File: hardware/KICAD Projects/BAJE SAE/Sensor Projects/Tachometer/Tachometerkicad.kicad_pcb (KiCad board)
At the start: 2 copper layers, 81 x 89 mm, 26 parts, among them J1 Conn_01x02, J3 Conn_01x02, J4 CAN to outer connector, Q1 NPN, U1 NE555P, U2 LM311

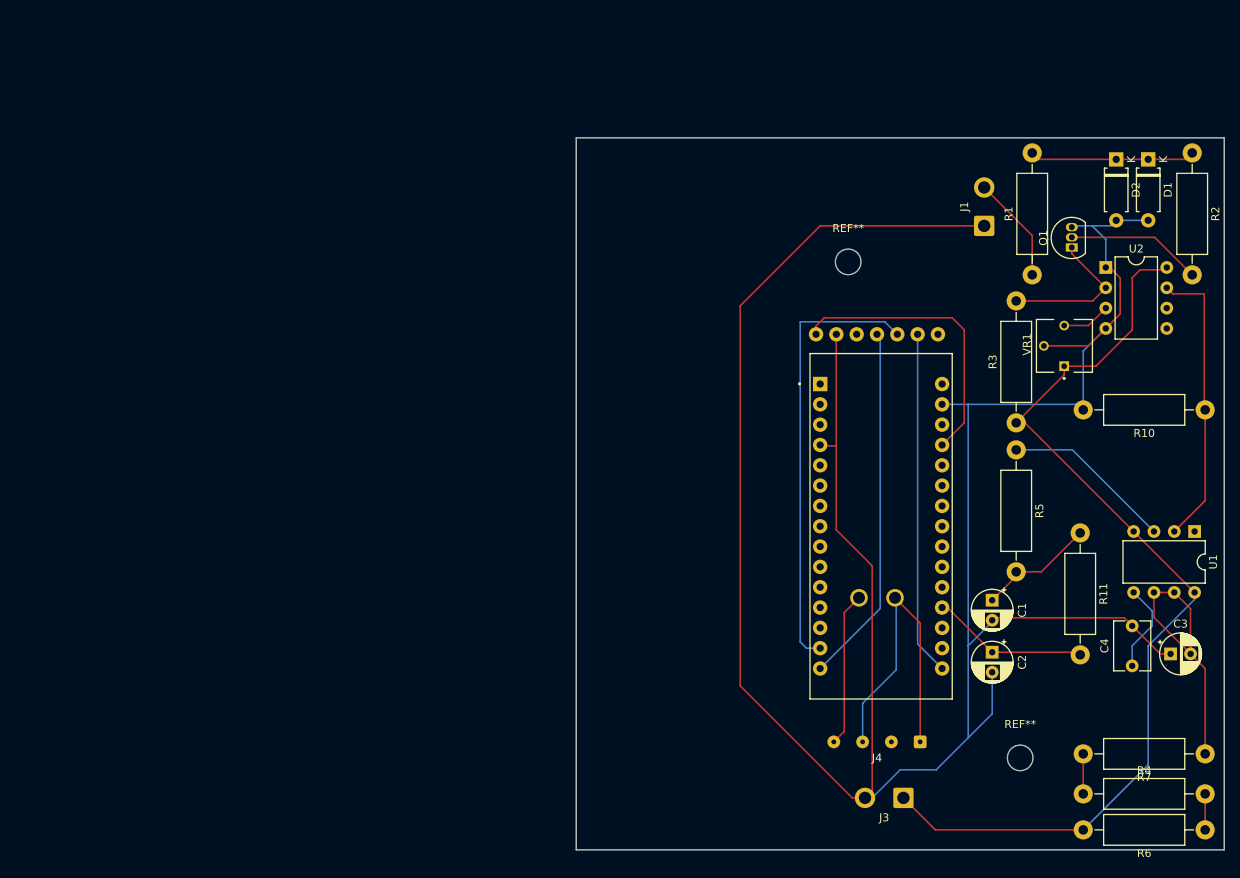
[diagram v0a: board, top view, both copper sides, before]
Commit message: Tach Update
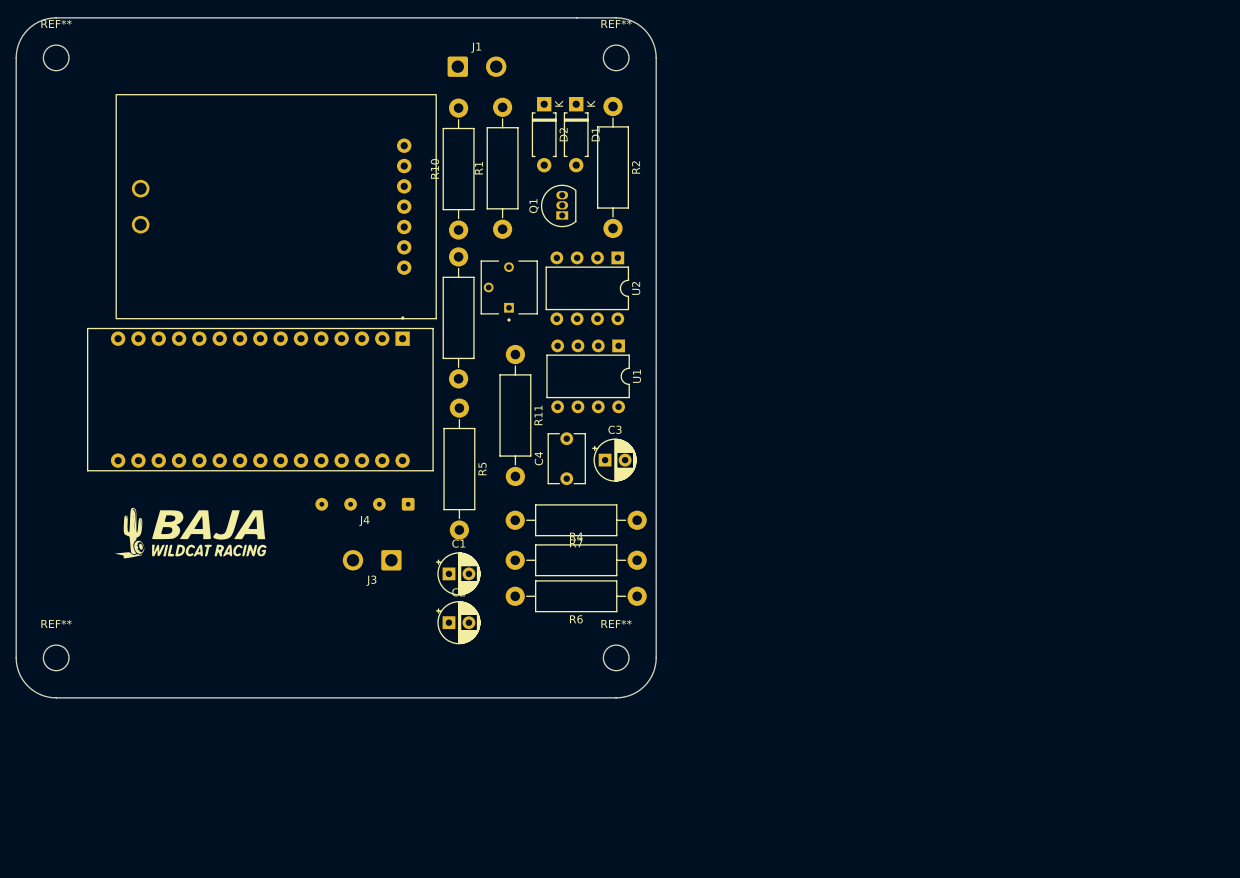
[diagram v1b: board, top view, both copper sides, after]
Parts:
- added G***: LOGO, BAJA SAE:Baja Logo, F.Cu at (56.8, 104.4)
- added REF**: MountingHole_3.2mm_M3, MountingHole:MountingHole_3.2mm_M3, F.Cu at (40.0, 120.0)
- added REF**: MountingHole_3.2mm_M3, MountingHole:MountingHole_3.2mm_M3, F.Cu at (40.0, 45.0)
- UNIT_2: moved to F.Cu
- moved R10 96.0 mm to (90.3, 66.5), turned to 90 degrees
- moved UNIT_1 79.2 mm to (65.5, 87.7), turned to -90 degrees
- moved UNIT_2 76.9 mm to (73.5, 61.2), turned to 180 degrees
- moved R4 76.8 mm to (97.4, 107.8)
- moved R6 76.8 mm to (112.6, 112.3)
- moved R7 76.8 mm to (112.6, 102.8)
- moved U1 75.6 mm to (110.3, 81.0)
- moved C3 74.7 mm to (108.6, 95.3)
- moved C4 74.5 mm to (103.8, 97.6)
- moved R11 74.0 mm to (97.4, 82.1)
- moved R2 72.6 mm to (109.6, 51.1)
- moved D1 71.8 mm to (105.0, 50.8)
- moved D2 71.8 mm to (101.0, 50.8)
- moved J3 70.6 mm to (81.9, 107.8)
- moved J4 70.6 mm to (84.0, 100.8)
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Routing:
- net GND: track 325.5 -> 0.00 mm
- net +5v: track 122.0 -> 0.00 mm
- net SI: track 55.6 -> 0.00 mm
- net SO: track 45.1 -> 0.00 mm
- net SCK: track 43.0 -> 0.00 mm
- net Low: track 39.1 -> 0.00 mm
- net 555 input: track 36.3 -> 0.00 mm
- net +5V: track 36.1 -> 0.00 mm
- net Net-(U1-DIS): track 33.9 -> 0.00 mm
- net 555 output: track 21.4 -> 0.00 mm
- net Net-(D1-K): track 20.7 -> 0.00 mm
- net arduino input: track 19.7 -> 0.00 mm
- net High: track 19.3 -> 0.00 mm
- net Comparator input: track 18.7 -> 0.00 mm
- net Net-(Q1-B): track 17.0 -> 0.00 mm
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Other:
- board size 81 x 89 mm -> 80 x 85 mm
- board text added: "Designed by Dylan Correa in Tucson, AZ"
- board text added: "Tachometer"
